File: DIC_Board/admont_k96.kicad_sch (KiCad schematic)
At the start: 8 parts, among them J34 0430450400, U35 TPS27S100APWPR

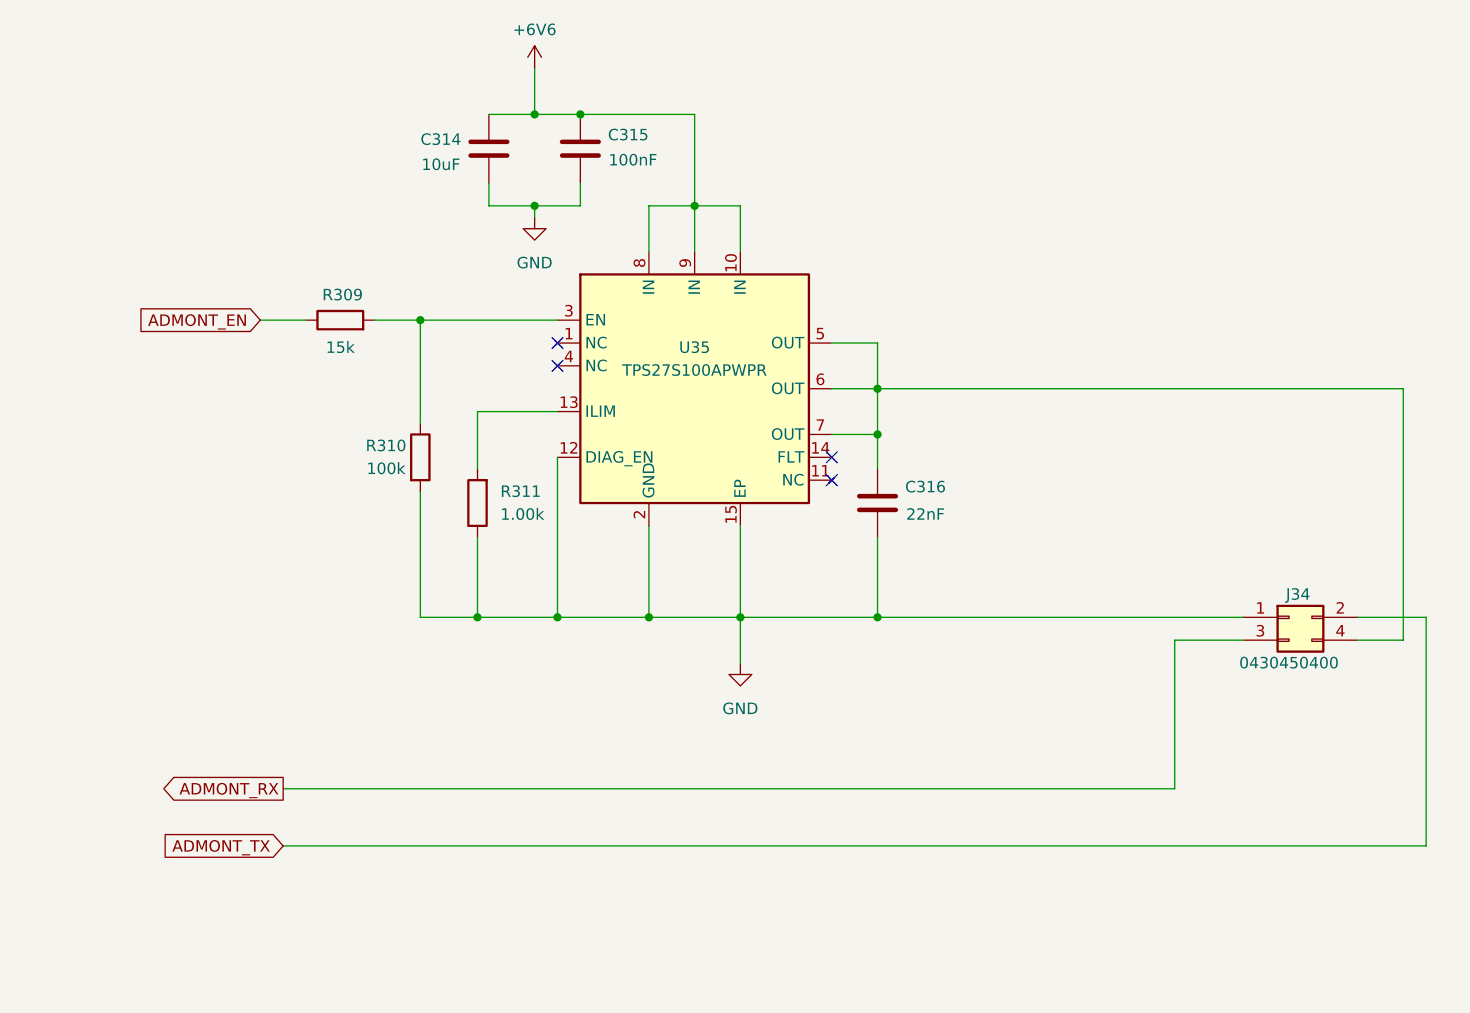
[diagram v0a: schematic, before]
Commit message: Checkpoint current schematic state
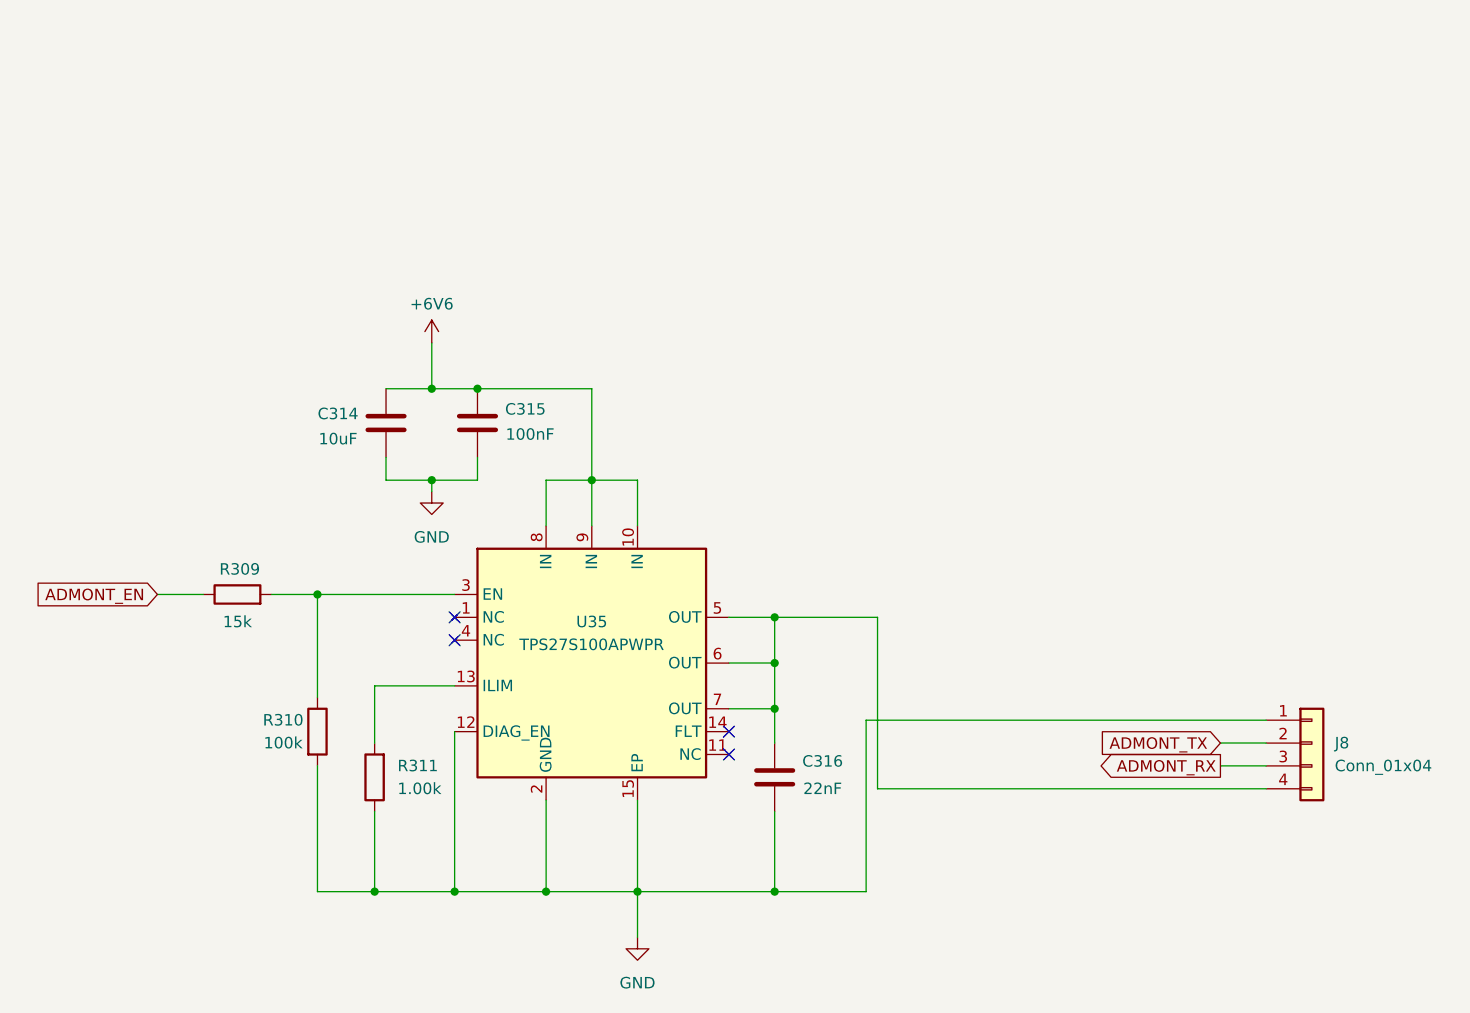
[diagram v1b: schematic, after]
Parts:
- removed J34: 0430450400, Connector_Molex:Molex_Micro-Fit_3.0_43045-0400_2x02_P3.00mm_Horizontal, symbol Connector_Generic:Conn_02x02_Odd_Even
- added J8: Conn_01x04, symbol Connector_Generic:Conn_01x04
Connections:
- net ADMONT_RX: now also J8.3 (Pin_3)
- net ADMONT_TX: now also J8.2 (Pin_2)
- net GND: now also J8.1 (Pin_1)
- net at C316.1, U35.5 (OUT), U35.6 (OUT)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: now also J8.4 (Pin_4)
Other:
- moved on the sheet: C314, C315, C316, R309, R310, R311, U35
